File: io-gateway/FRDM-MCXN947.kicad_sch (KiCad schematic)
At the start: 2 parts

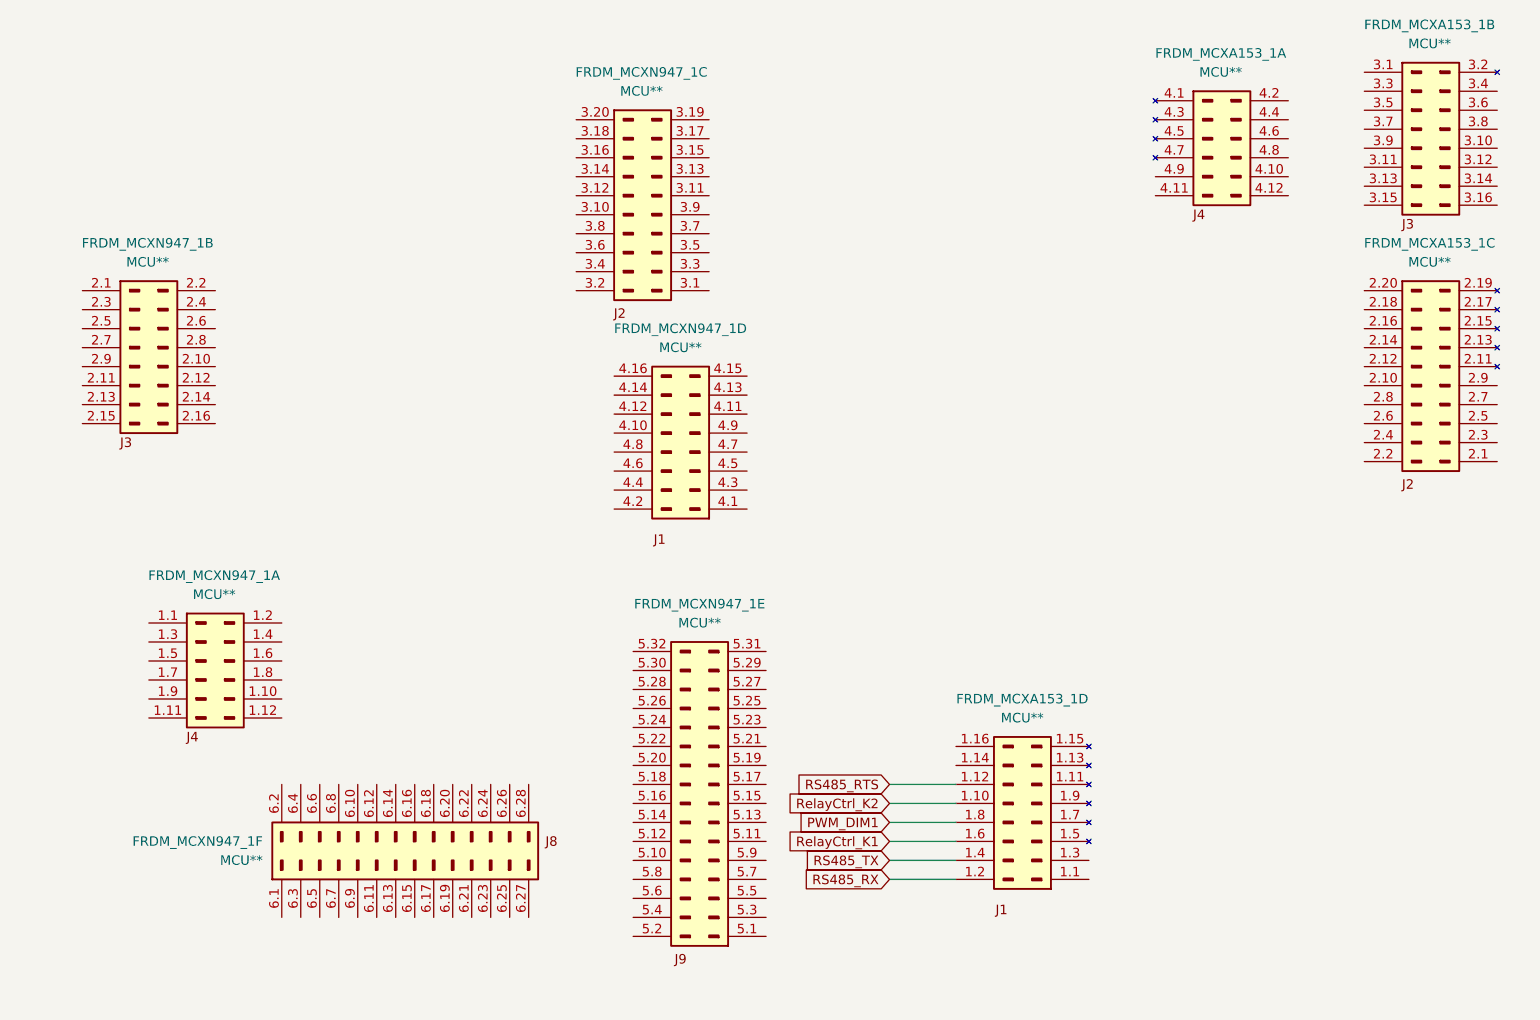
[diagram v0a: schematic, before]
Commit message: layout for first dimmer
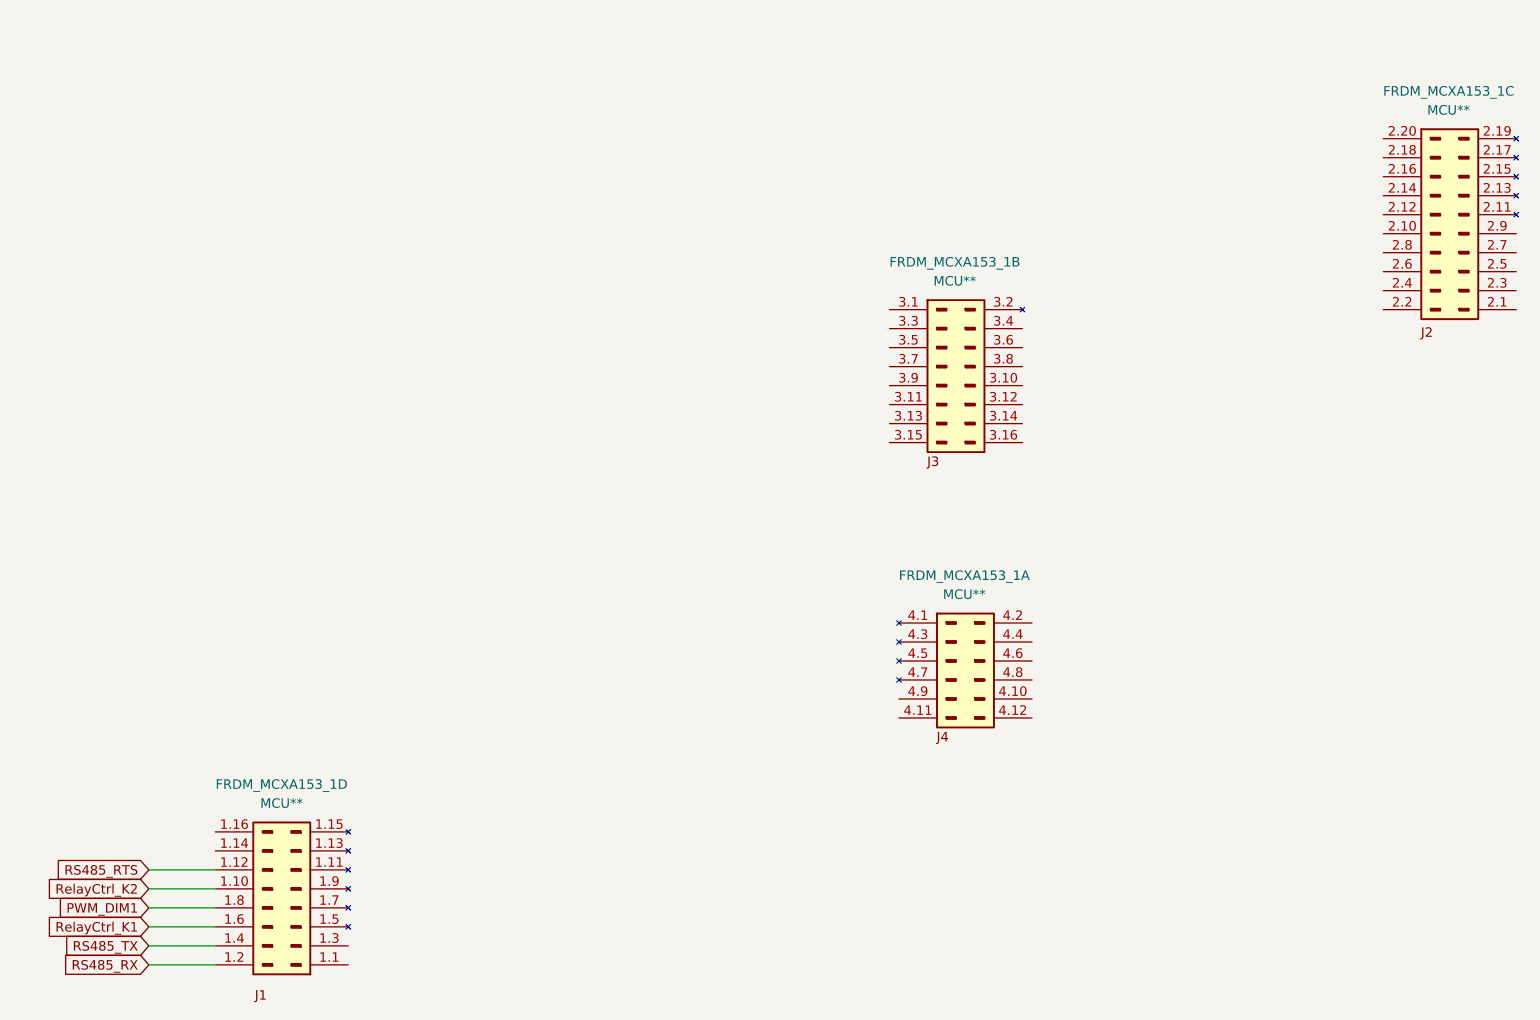
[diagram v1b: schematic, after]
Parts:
- removed FRDM_MCXN947_1: MCU**, FRDM-MCXN947:FRDM-MCXN947, symbol FRDM-MCXN947__Shield_Template-altium-import:MCU**
- FRDM_MCXA153_1: now in the parts list
